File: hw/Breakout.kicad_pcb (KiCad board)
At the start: 2 copper layers, 22.8 x 27.4 mm, 7 parts, among them J1 ST60X-18S30, J2 SJ-3523-SMT-TR, J3 BM03B-SRSS-TBT_LF__SN_, U1 12401610E4-2A

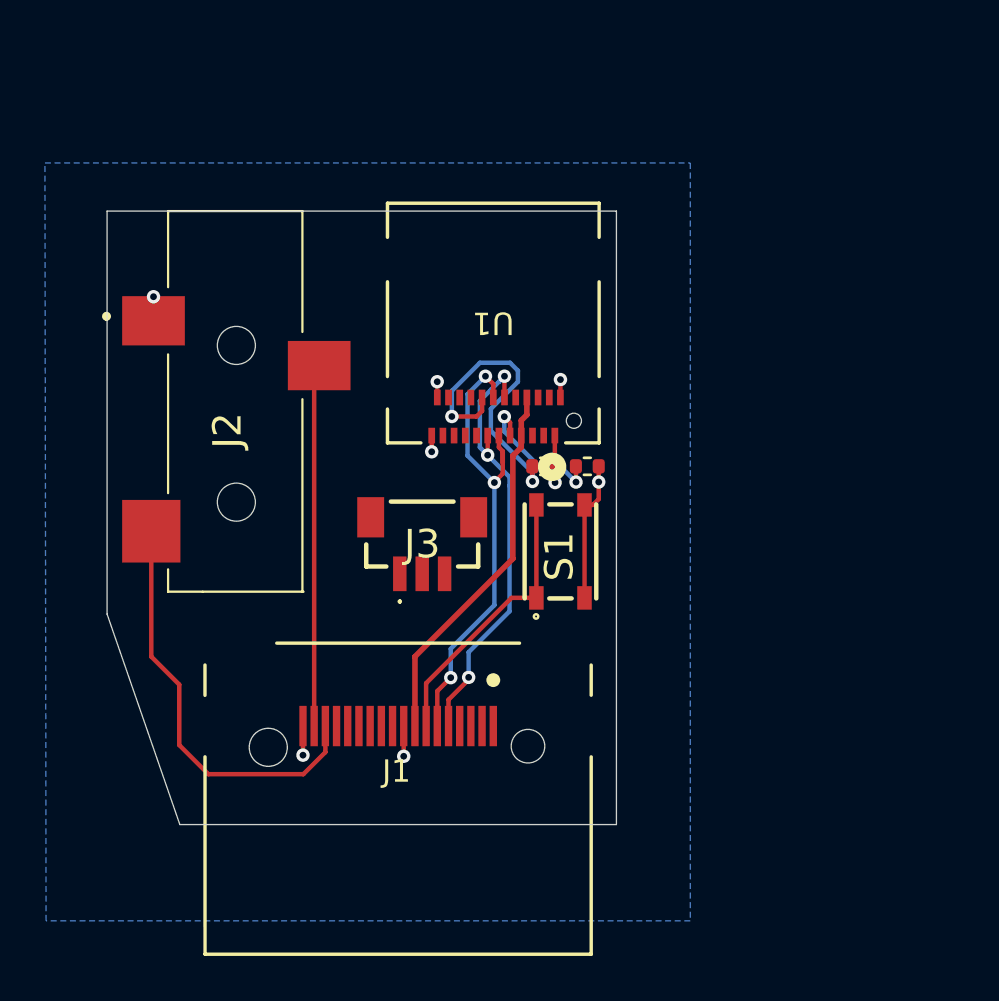
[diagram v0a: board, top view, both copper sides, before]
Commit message: Work in progress
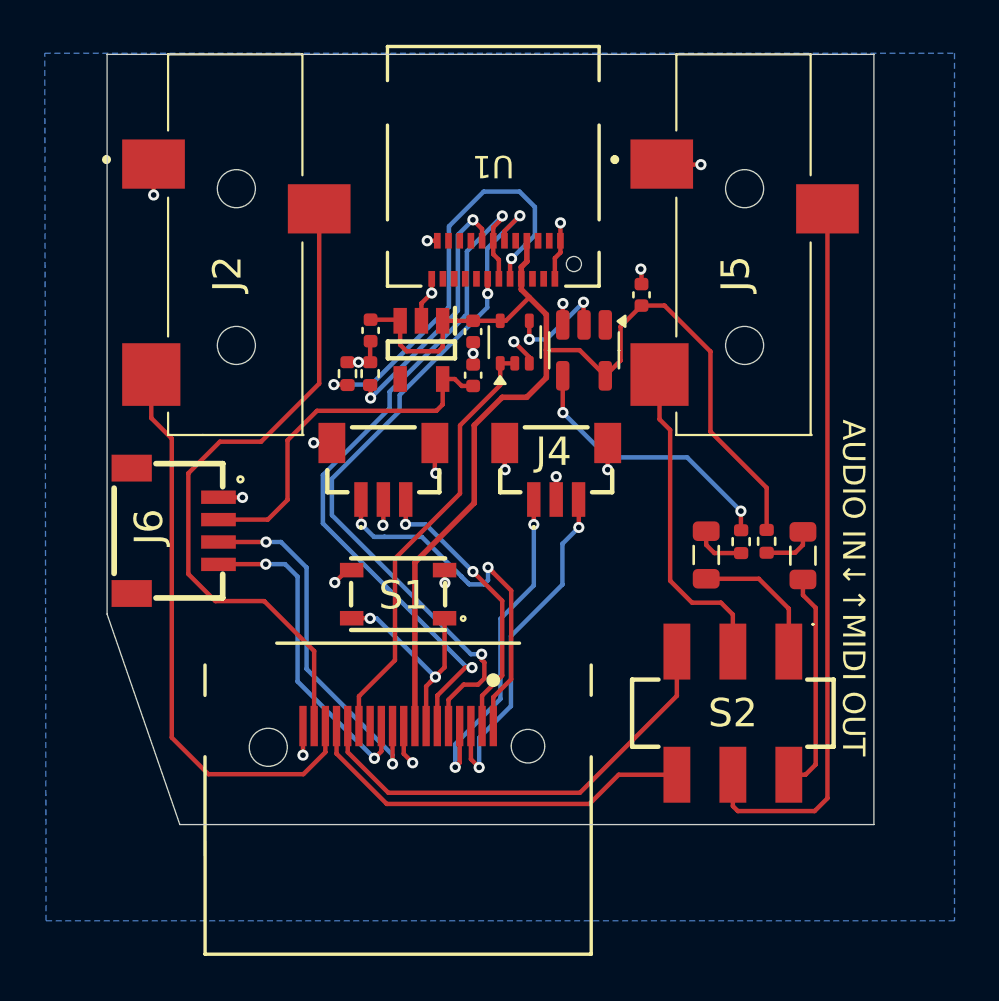
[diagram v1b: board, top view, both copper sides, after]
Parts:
- added C1: 0.1uF, Capacitor_SMD:C_0402_1005Metric, F.Cu at (106.6, 80.7)
- added C2: 0.1uF, Capacitor_SMD:C_0402_1005Metric, F.Cu at (99.1, 82.4)
- added C3: 1uF, Capacitor_SMD:C_0402_1005Metric, F.Cu at (99.1, 84.3)
- added C5: 0.1uF, Capacitor_SMD:C_0402_1005Metric, F.Cu at (94.5, 82.3)
- added FB1: 1KΩ@100MHz, Inductor_SMD:L_0805_2012Metric, F.Cu at (109.5, 92.4)
- added FB2: 1KΩ@100MHz, Inductor_SMD:L_0805_2012Metric, F.Cu at (113.8, 92.4)
- added IC1: AP2112K-3.3TRG1, BreakoutLibrary:SOT95P285X140-5N, F.Cu at (96.8, 83.2)
- added J4: BM03B-SRSS-TBT_LF__SN_, BreakoutLibrary:BM03BSRSSTBTLFSN, F.Cu at (102.8, 88.3)
- added J5: SJ-3523-SMT-TR, BreakoutLibrary:SJ3523SMTTR, F.Cu at (111.2, 72.5)
- added J6: SM04B-SRSS-TB_LF__SN_, BreakoutLibrary:SM04B-SRSS-TB_LFSN_, F.Cu at (83.1, 88.3)
- added R3: 220, Resistor_SMD:R_0402_1005Metric, F.Cu at (111.1, 91.8)
- added R4: 220, Resistor_SMD:R_0402_1005Metric, F.Cu at (112.2, 91.8)
- added S2: JS202011SCQN, BreakoutLibrary:JS202011SCQN, F.Cu at (110.7, 99.4)
- added U2: 74LVC1G00, Package_TO_SOT_SMD:SOT-353_SC-70-5, F.Cu at (101.0, 82.8)
- added U3: 74LVC1G06, Package_TO_SOT_SMD:TSOT-23-5, F.Cu at (104.1, 83.2)
- moved R1 11.5 mm to (93.5, 84.3), turned to -90 degrees
- moved R2 8.79 mm to (94.5, 84.3), turned to -90 degrees
- moved S1 7.50 mm to (95.8, 94.1), turned to 180 degrees
- moved J2 7.00 mm to (88.5, 72.5)
- moved U1 7.00 mm to (100.0, 75.0)
- moved J3 3.74 mm to (95.1, 88.3)
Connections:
- net Net-(J2-RING) renamed /HP_R
- net Net-(J2-TIP) renamed /HP_L
- J1 pad 1: /SWCLK -> SWCLK
- J1 pad 10: /I2C0_SDA -> I2C0_SDA
- J1 pad 11: /I2C0_SDL -> I2C0_SDL
- J1 pad 13: /UART1_TX -> UART1_TX
- J1 pad 14: unconnected-(J1-Pad14) -> IN2_L
- J1 pad 15: unconnected-(J1-Pad15) -> IN2_R
- J1 pad 2: /SWDIO -> SWD
- J1 pad 3: /UART0_TX -> UART0_TX
- J1 pad 4: /UART0_RX -> UART0_RX
- J3 pad 1: unconnected-(J3-Pad1) -> SWCLK
- J3 pad 2: unconnected-(J3-Pad2) -> GND
- J3 pad 3: unconnected-(J3-Pad3) -> SWD
- J3 pad 4: unconnected-(J3-MP1-Pad4) -> GND
- J3 pad 5: unconnected-(J3-MP2-Pad5) -> GND
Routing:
- net USB_VBUS: track 16.7 -> 55.2 mm
- net J5_RING: track 0.00 -> 32.3 mm
- net IN2_L: track 0.00 -> 20.4 mm
- net UART1_TX: track 0.00 -> 19.5 mm
- net IN2_R: track 0.00 -> 17.9 mm
- net SWCLK: track 0.00 -> 16.7 mm, vias 0 -> 2
- net I2C0_SDA: track 0.00 -> 16.5 mm, vias 0 -> 2
- net +3.3V: track 0.00 -> 16.3 mm
- net UART0_TX: track 0.00 -> 15.8 mm, vias 0 -> 2
- net UART0_RX: track 0.00 -> 15.3 mm, vias 0 -> 2
- net I2C0_SDL: track 0.00 -> 14.9 mm, vias 0 -> 2
- net /HP_R: track 15.7 -> 30.2 mm
- net J5_TIP: track 0.00 -> 14.5 mm
- net USB_D-: track 19.6 -> 32.6 mm
- net SWD: track 0.00 -> 12.8 mm, vias 0 -> 2
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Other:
- board size 22.8 x 27.4 mm -> 34.2 x 34.4 mm
- board text added: "AUDIO IN↓↑MIDI OUT"
